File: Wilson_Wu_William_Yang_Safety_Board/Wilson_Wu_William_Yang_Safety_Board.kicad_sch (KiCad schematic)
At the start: 17 parts, among them J1 22035035, J2 XT60-M, J3 XT60-M, J4 M22-7130442, J5 Molex Micro-Fit 4 Pin, J6 430450200, J7 430450200, K1 Fujitsu_FTR-LYAA005x, Q1 IRLML6344TRPBF, U2 MCP2562-E/P, U3 MCP6286T-E/OT, U4 4002, U5 100 ohm

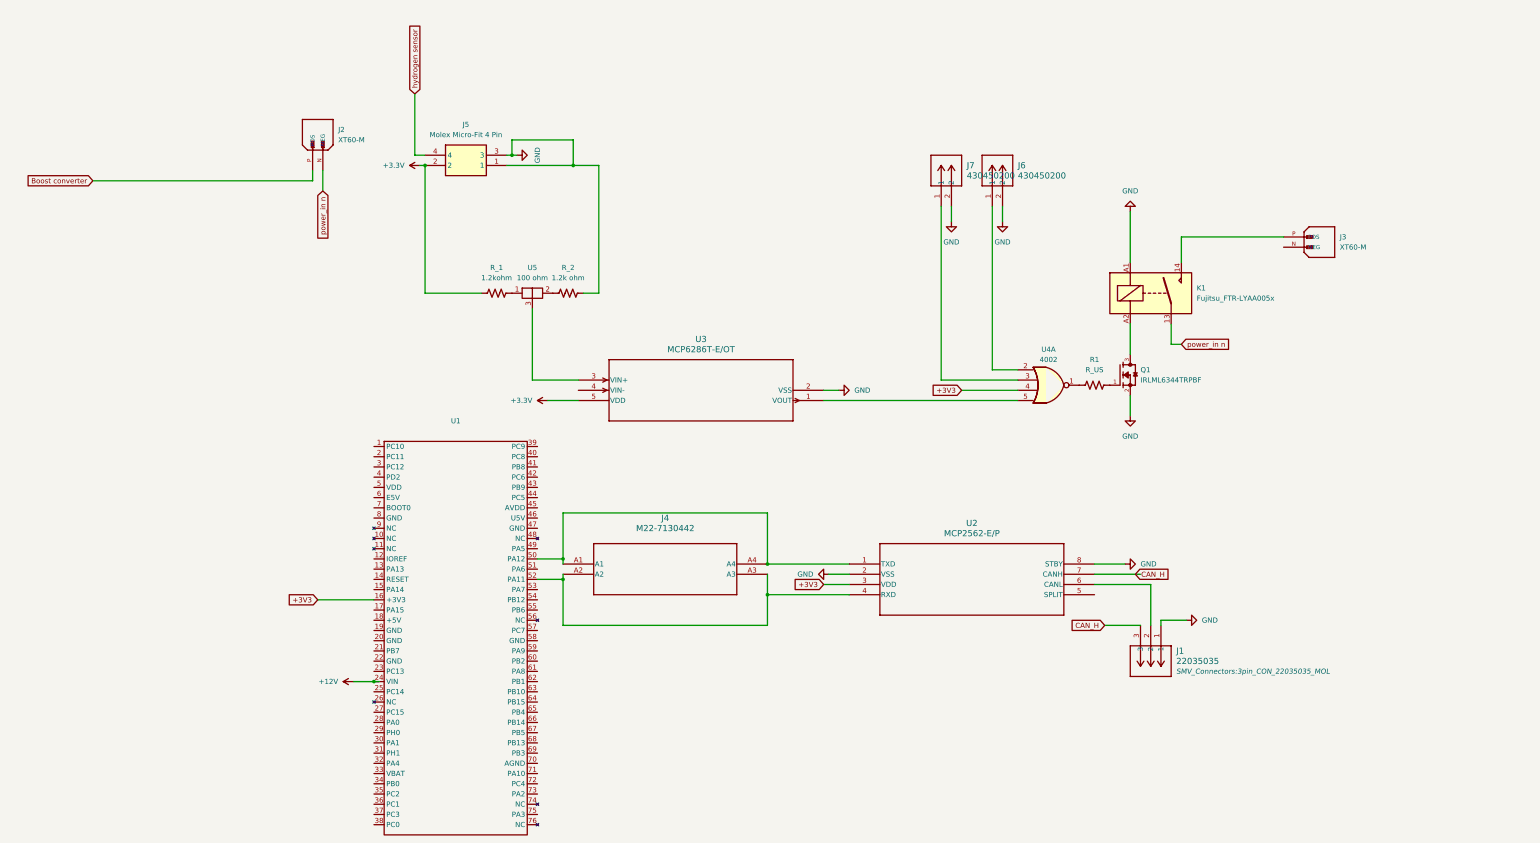
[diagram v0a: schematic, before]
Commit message: edited board
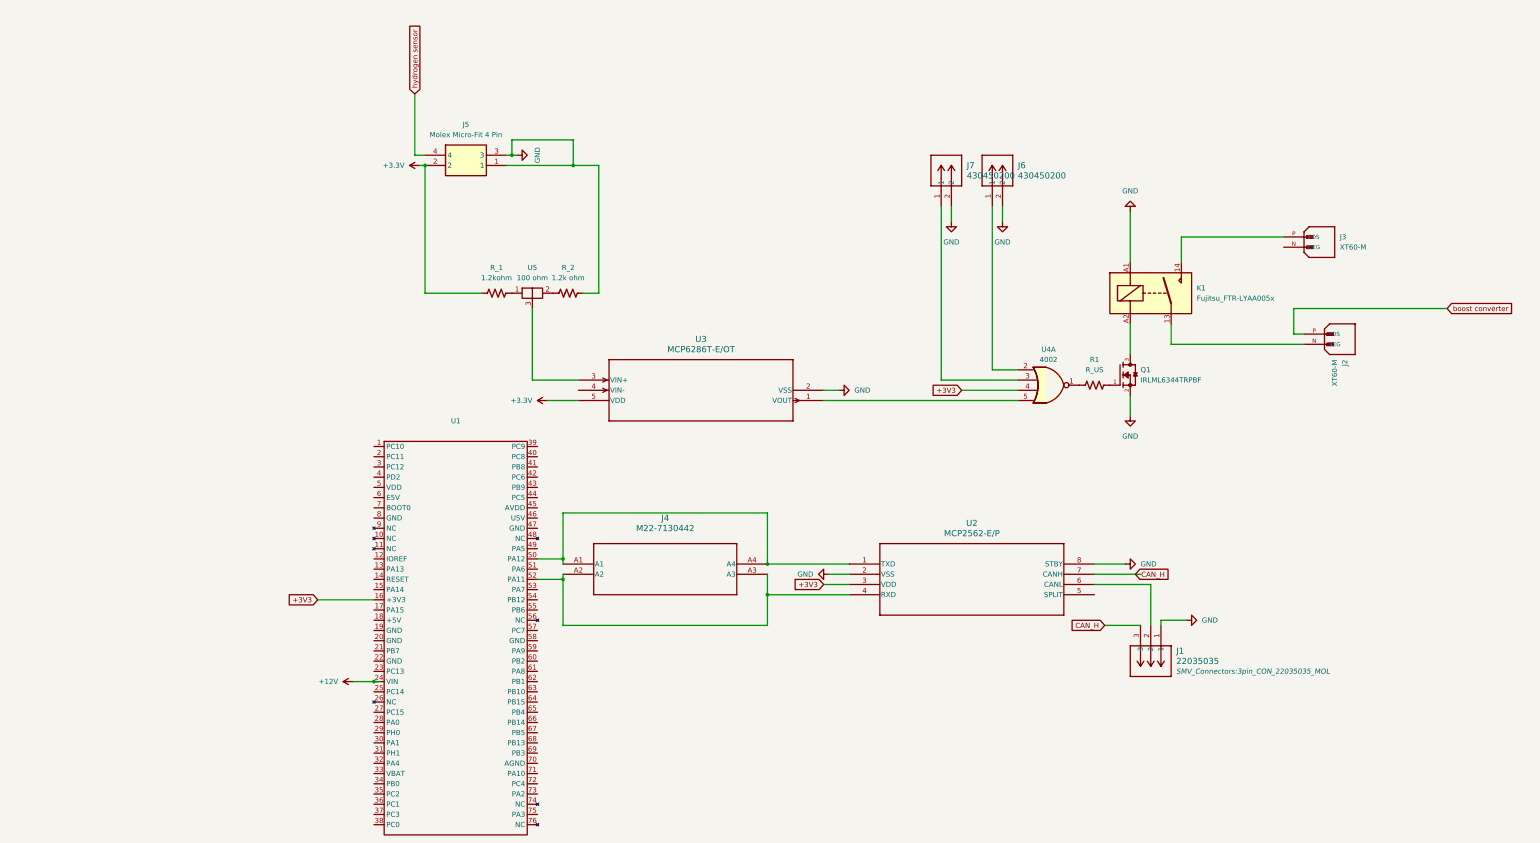
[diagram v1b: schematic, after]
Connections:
- net Boost converter renamed boost converter
- net power_in n: no longer names the net of J2.N (NEG), K1.13
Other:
- moved on the sheet: J2
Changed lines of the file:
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@@
 	(wire
 		(pts
-			(xy 21.59 29.21) (xy 21.59 26.67)
+			(xy 265.43 67.31) (xy 267.97 67.31)
 		)
 		(stroke
@@
 	(wire
 		(pts
-			(xy -33.02 29.21) (xy 21.59 29.21)
-		)
-		(stroke
-			(width 0)
-			(type default)
-		)
-	)
-	(wire
-		(pts
 			(xy 182.88 81.28) (xy 196.85 81.28)
 		)
@@
 	(wire
 		(pts
-			(xy 24.13 26.67) (xy 24.13 31.75)
-		)
-		(stroke
-			(width 0)
-			(type default)
-		)
-	)
-	(wire
-		(pts
 			(xy 69.85 22.86) (xy 71.12 22.86)
 		)
@@
 	(wire
 		(pts
+			(xy 265.43 60.96) (xy 303.53 60.96)
+		)
+		(stroke
+			(width 0)
+			(type default)
+		)
+	)
+	(wire
+		(pts
 			(xy 69.85 25.4) (xy 86.36 25.4)
 		)
@@
 	(wire
 		(pts
-			(xy 234.95 69.85) (xy 237.49 69.85)
+			(xy 234.95 69.85) (xy 267.97 69.85)
 		)
 		(stroke
@@
 		(pts
 			(xy 180.34 35.56) (xy 180.34 39.37)
+		)
+		(stroke
+			(width 0)
+			(type default)
+		)
+	)
+	(wire
+		(pts
+			(xy 265.43 67.31) (xy 265.43 60.96)
 		)
 		(stroke
@@
 		)
 	)
-	(global_label "Boost converter"
-		(shape input)
-		(at -33.02 29.21 180)
-		(fields_autoplaced yes)
-		(effects
-			(font
-				(size 1.27 1.27)
-			)
-			(justify right)
-		)
-		(property "Intersheetrefs" "${INTERSHEET_REFS}"
-			(at -51.1241 29.21 0)
-			(effects
-				(font
-					(size 1.27 1.27)
-				)
-				(justify right)
-				(hide yes)
-			)
-		)
-	)
 	(global_label "CAN_H"
 		(shape input)
@@
 		)
 	)
-	(global_label "power_in n"
+	(global_label "boost converter"
 		(shape input)
-		(at 237.49 69.85 0)
+		(at 303.53 60.96 0)
 		(fields_autoplaced yes)
 		(effects
@@
 		)
 		(property "Intersheetrefs" "${INTERSHEET_REFS}"
-			(at 250.8165 69.85 0)
+			(at 321.5131 60.96 0)
 			(effects
 				(font
@@
 				)
 				(justify left)
-				(hide yes)
-			)
-		)
-	)
-	(global_label "power_in n"
-		(shape input)
-		(at 24.13 31.75 270)
-		(fields_autoplaced yes)
-		(effects
-			(font
-				(size 1.27 1.27)
-			)
-			(justify right)
-		)
-		(property "Intersheetrefs" "${INTERSHEET_REFS}"
-			(at 24.13 45.0765 90)
-			(effects
-				(font
-					(size 1.27 1.27)
-				)
-				(justify right)
 				(hide yes)
 			)
@@
 	(symbol
 		(lib_id "SMV_Custom:XT60-M")
-		(at 24.13 21.59 90)
+		(at 273.05 69.85 0)
 		(unit 1)
 		(exclude_from_sim no)
@@
 		(fields_autoplaced yes)
 		(property "Reference" "J2"
-			(at 27.94 16.5099 90)
+			(at 278.1301 73.66 90)
 			(effects
 				(font
@@
 		)
 		(property "Value" "XT60-M"
-			(at 27.94 19.0499 90)
+			(at 275.5901 73.66 90)
 			(effects
 				(font
@@
 		)
 		(property "Footprint" "SMV_Connectors:AMASS_XT60-M"
-			(at 24.13 21.59 0)
+			(at 273.05 69.85 0)
 			(effects
 				(font
@@
 		)
 		(property "Datasheet" ""
-			(at 24.13 21.59 0)
+			(at 273.05 69.85 0)
 			(effects
 				(font
@@
 		)
 		(property "Description" ""
-			(at 24.13 21.59 0)
+			(at 273.05 69.85 0)
 			(effects
 				(font
@@
 		)
 		(property "MF" "AMASS"
-			(at 24.13 21.59 0)
+			(at 273.05 69.85 0)
 			(effects
 				(font
@@
 		)
 		(property "MAXIMUM_PACKAGE_HEIGHT" "16.00 mm"
-			(at 24.13 21.59 0)
+			(at 273.05 69.85 0)
 			(effects
 				(font
@@
 		)
 		(property "Package" "Package"
-			(at 24.13 21.59 0)
+			(at 273.05 69.85 0)
 			(effects
 				(font
@@
 		)
 		(property "Price" "None"
-			(at 24.13 21.59 0)
+			(at 273.05 69.85 0)
 			(effects
 				(font
@@
 		)
 		(property "Check_prices" "https://www.snapeda.com/parts/XT60-M/AMASS/view-part/?ref=eda"
-			(at 24.13 21.59 0)
+			(at 273.05 69.85 0)
 			(effects
 				(font
@@
 		)
 		(property "STANDARD" "IPC 7351B"
-			(at 24.13 21.59 0)
+			(at 273.05 69.85 0)
 			(effects
 				(font
@@
 		)
 		(property "PARTREV" "V1.2"
-			(at 24.13 21.59 0)
+			(at 273.05 69.85 0)
 			(effects
 				(font
@@
 		)
 		(property "SnapEDA_Link" "https://www.snapeda.com/parts/XT60-M/AMASS/view-part/?ref=snap"
-			(at 24.13 21.59 0)
+			(at 273.05 69.85 0)
 			(effects
 				(font
@@
 		)
 		(property "MP" "XT60-M"
-			(at 24.13 21.59 0)
+			(at 273.05 69.85 0)
 			(effects
 				(font
@@
 		)
 		(property "Description_1" "\n                        \n                            Plug; DC supply; XT60; male; PIN: 2; for cable; soldered; 30A; 500V\n                        \n"
-			(at 24.13 21.59 0)
+			(at 273.05 69.85 0)
 			(effects
 				(font
@@
 		)
 		(property "Availability" "Not in stock"
-			(at 24.13 21.59 0)
+			(at 273.05 69.85 0)
 			(effects
 				(font
@@
 		)
 		(property "MANUFACTURER" "AMASS"
-			(at 24.13 21.59 0)
-			(effects
-				(font
+			(at 273.05 69.85 0)
+			(effects
+				(font
